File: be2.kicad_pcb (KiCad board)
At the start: 2 copper layers, 50 x 62.5 mm, 56 parts, among them K1 CONN_01X03, K2 CONN_01X02, K3 CONN_01X01, K4 CONN_01X03, K5 CONN_01X01, U1 AD620A, U100 LM311N, U101 LM311N, U102 LM311N, U103 LM311N, U2 TL082, U3 TL082, U4 TL082

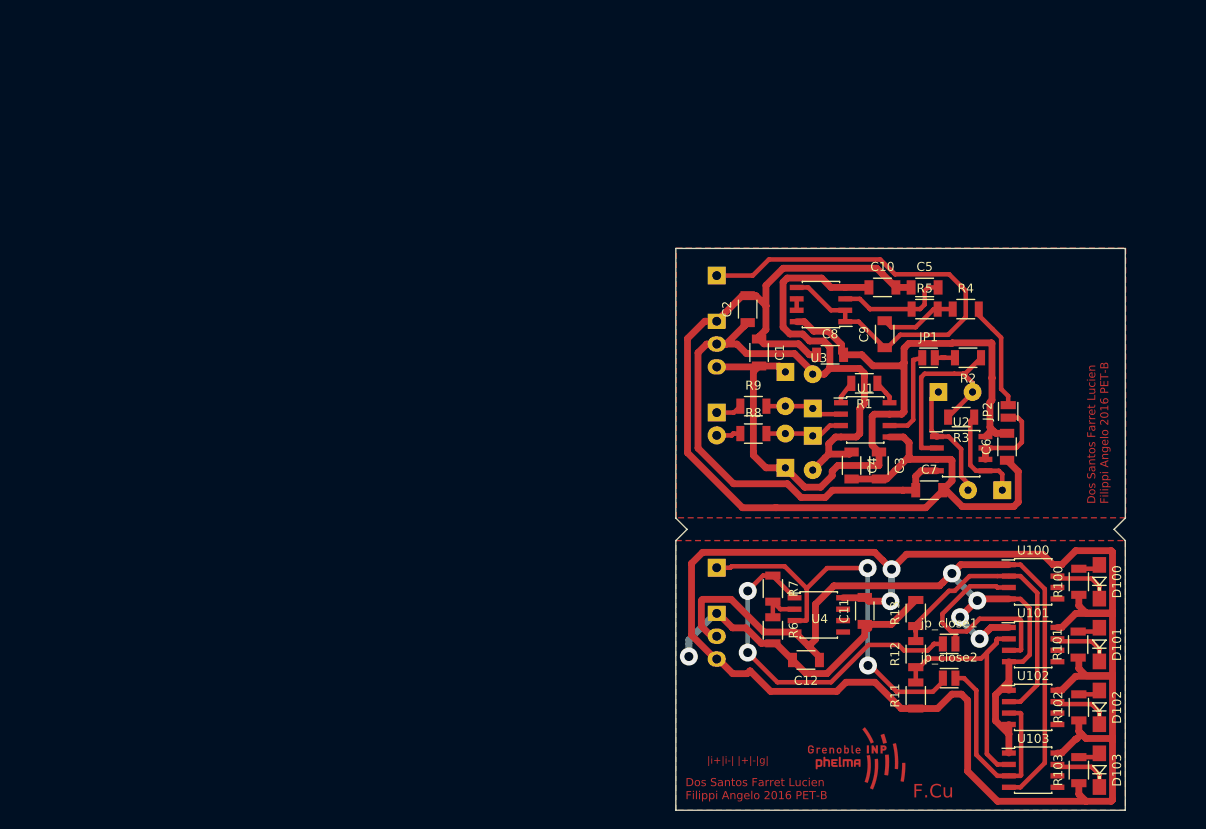
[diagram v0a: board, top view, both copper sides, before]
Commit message: mechanical drawing
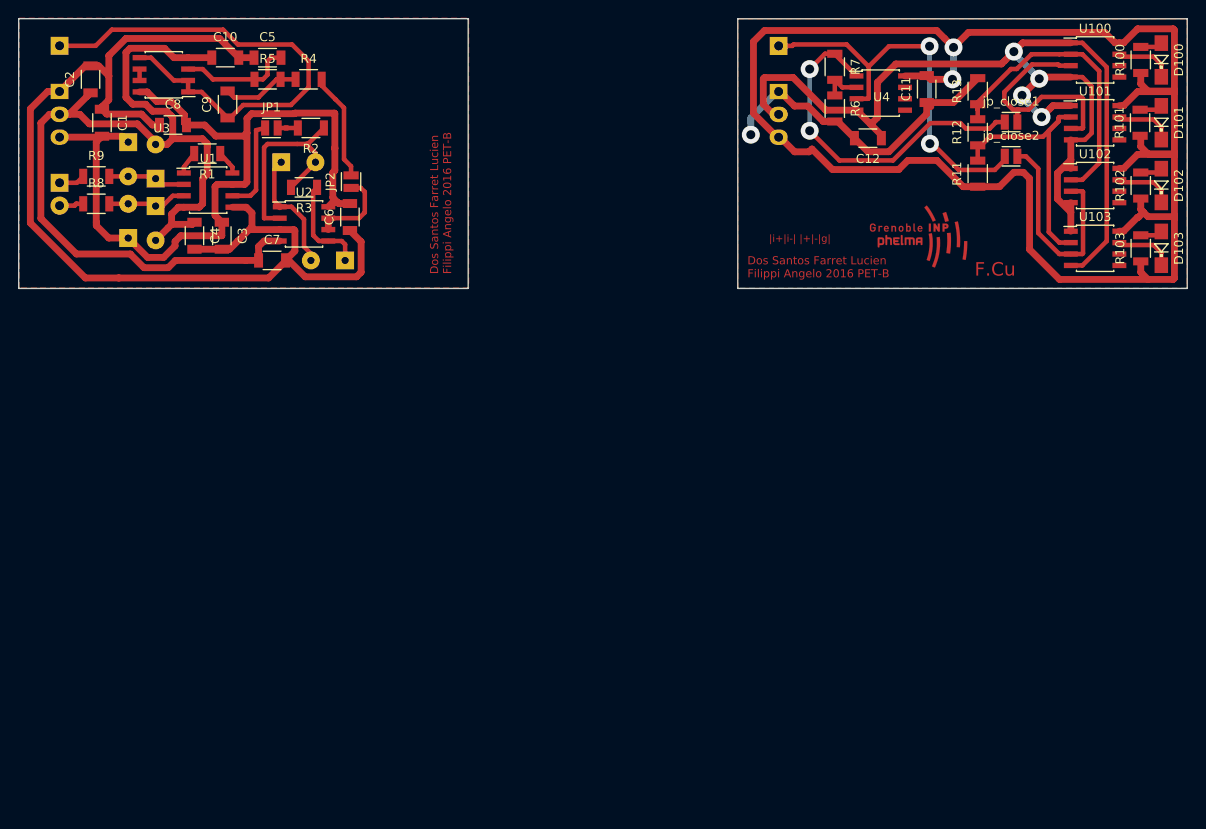
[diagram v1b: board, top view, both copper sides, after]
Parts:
- moved C1 77.4 mm to (53.1, 49.5)
- moved C7 77.4 mm to (72.0, 64.8)
- moved JP2 77.4 mm to (80.8, 56.0)
- moved R4 77.4 mm to (76.1, 44.6)
- moved R5 77.4 mm to (71.5, 44.6)
- moved U1 77.4 mm to (64.9, 57.0)
- moved C10 77.4 mm to (66.8, 42.2)
- moved C2 77.4 mm to (51.8, 44.6)
- moved C3 77.4 mm to (66.4, 62.0)
- moved C4 77.4 mm to (63.4, 62.0)
- moved C5 77.4 mm to (71.5, 42.2)
- moved C6 77.4 mm to (80.7, 60.0)
- moved C8 77.4 mm to (61.0, 49.7)
- moved D1 77.4 mm to (73.0, 53.9)
- moved D2 77.4 mm to (80.1, 64.8)
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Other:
- board size 50 x 62.5 mm -> 130 x 30 mm
- board text added: "+15v [4]"
- board text added: "-15v [3]"
- board text added: "KA-001 module"
- board text added: "KA-002 module"
- board text added: "ground [2]"
- board text added: "in+ [5]"
- board text added: "in- [6]"
- board text added: "mean_in [1]"
- board text added: "mean_out [1]"
